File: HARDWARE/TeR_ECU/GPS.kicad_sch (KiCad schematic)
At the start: 11 parts, among them J5 GPS_ANT, U10 NEO-M9N

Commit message: Began layout
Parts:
- J5: footprint (none) -> Connector_Coaxial:SMA_Amphenol_132289_EdgeMount
- L2: footprint (none) -> Inductor_SMD:L_0805_2012Metric
- R45, R46: footprint (none) -> Resistor_SMD:R_0603_1608Metric
- TP1: footprint (none) -> TestPoint:TestPoint_Pad_1.0x1.0mm
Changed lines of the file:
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@@
 			)
 		)
-		(property "Footprint" ""
+		(property "Footprint" "Inductor_SMD:L_0805_2012Metric"
 			(at 161.29 85.09 0)
 			(effects
@@
 			)
 		)
-		(property "Footprint" ""
+		(property "Footprint" "Resistor_SMD:R_0603_1608Metric"
 			(at 144.78 115.57 0)
 			(effects
@@
 			)
 		)
-		(property "Footprint" ""
+		(property "Footprint" "Connector_Coaxial:SMA_Amphenol_132289_EdgeMount"
 			(at 191.77 92.71 0)
 			(effects
@@
 			)
 		)
-		(property "Footprint" ""
+		(property "Footprint" "Resistor_SMD:R_0603_1608Metric"
 			(at 163.068 77.47 90)
 			(effects
@@
 			)
 		)
-		(property "Footprint" ""
+		(property "Footprint" "TestPoint:TestPoint_Pad_1.0x1.0mm"
 			(at 92.71 100.33 0)
 			(effects

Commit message: First layout prototype
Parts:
- D25: footprint LED_SMD:LED_0201_0603Metric -> LED_SMD:LED_0603_1608Metric
- D26: footprint SODFL1006X40N -> GPS_D:SODFL1006X40N
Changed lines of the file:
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@@
 			)
 		)
-		(property "Footprint" "SODFL1006X40N"
+		(property "Footprint" "GPS_D:SODFL1006X40N"
 			(at 67.64 102.87 0)
 			(effects
@@
 			)
 		)
-		(property "Footprint" "LED_SMD:LED_0201_0603Metric"
+		(property "Footprint" "LED_SMD:LED_0603_1608Metric"
 			(at 144.78 106.68 0)
 			(effects

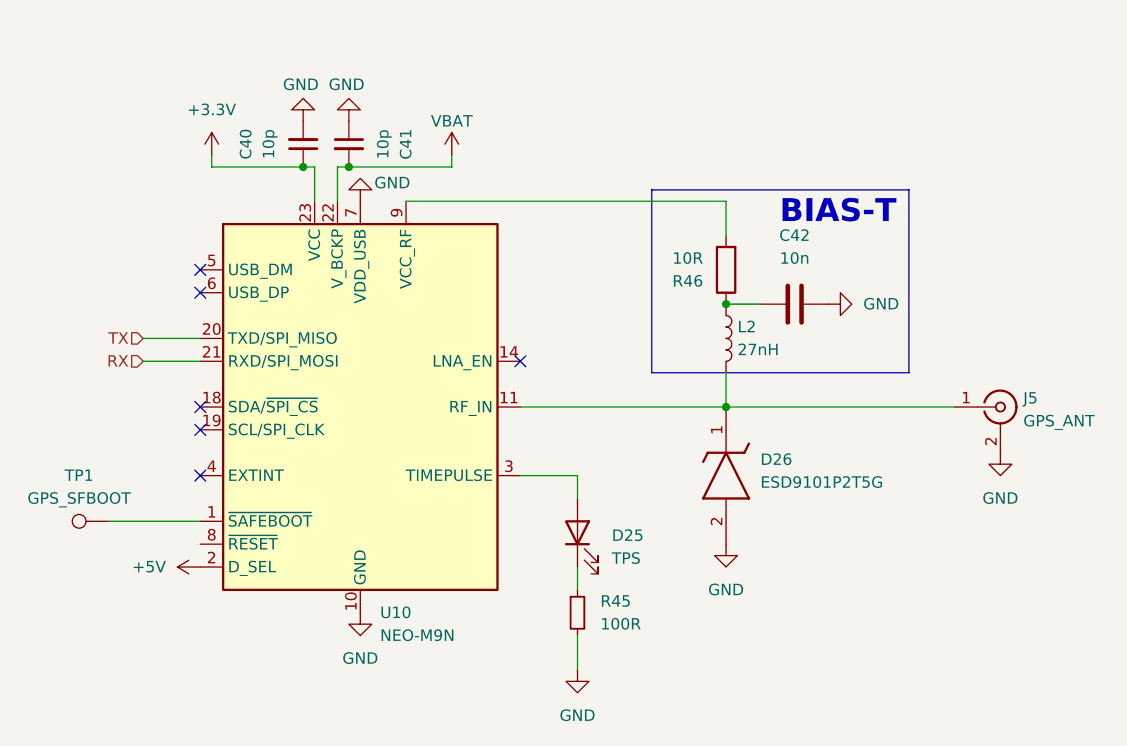
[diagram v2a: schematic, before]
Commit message: Finished layout, RF design, and quick DRC check, Lookin gud
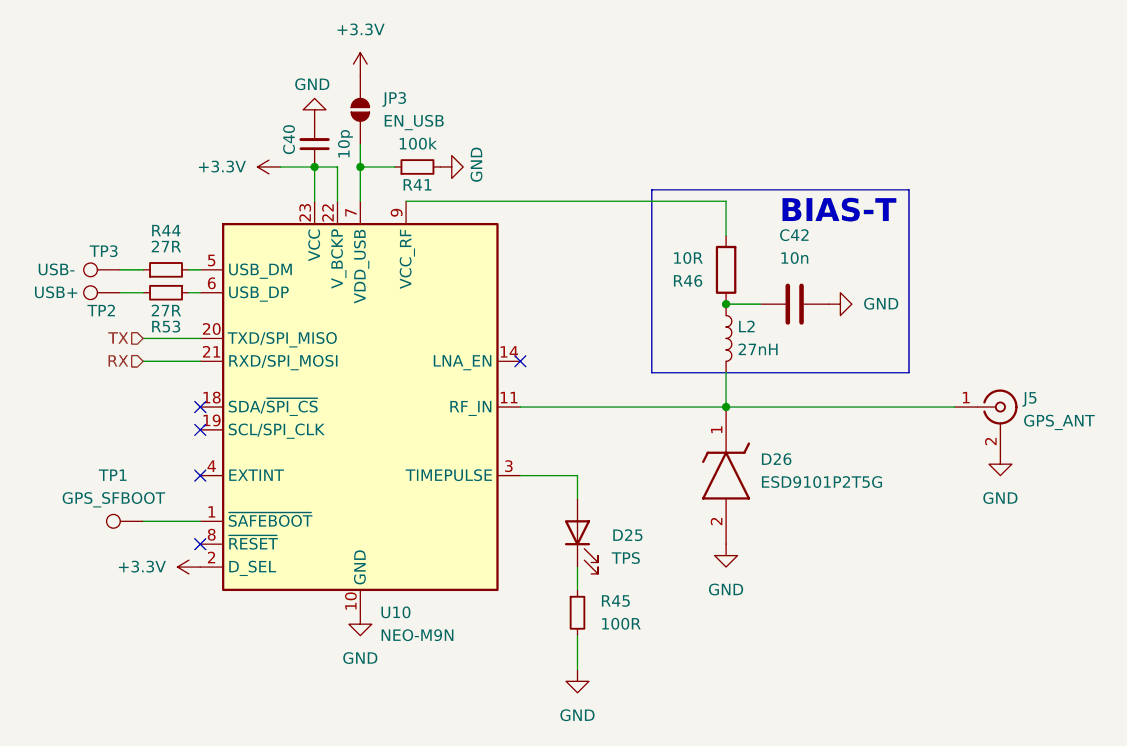
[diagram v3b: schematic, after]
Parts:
- removed C41: 10p, Capacitor_SMD:C_0603_1608Metric, symbol Device:C_Small
- added JP3: EN_USB, Jumper:SolderJumper-2_P1.3mm_Open_RoundedPad1.0x1.5mm, symbol Jumper:SolderJumper_2_Open
- added R41: 100k, Resistor_SMD:R_0603_1608Metric, symbol Device:R_Small
- added R44, R53: 27R, Resistor_SMD:R_0603_1608Metric, symbol Device:R_Small
- added TP2: USB+, TestPoint:TestPoint_Pad_1.0x1.0mm, symbol Connector:TestPoint
- added TP3: USB-, TestPoint:TestPoint_Pad_1.0x1.0mm, symbol Connector:TestPoint
- C42: footprint Capacitor_SMD:C_0603_1608Metric -> Capacitor_SMD:C_0402_1005Metric
- L2: footprint Inductor_SMD:L_0805_2012Metric -> Inductor_SMD:L_0402_1005Metric
- R46: footprint Resistor_SMD:R_0603_1608Metric -> Resistor_SMD:R_0402_1005Metric
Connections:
- net +5V is gone; now on net +3.3V: U10.2 (D_SEL)
- net VBAT is gone; now on net +3.3V: U10.22 (V_BCKP)
- net +3.3V: now also JP3.2 (B)
- net GND: now also R41.2; no longer U10.7 (VDD_USB)
- net at U10.5 (USB_DM): now also R44.2
- net at U10.6 (USB_DP): now also R53.1
- new net: R53.2, TP2.1
- new net: R44.1, TP3.1
- new net: JP3.1 (A), R41.1, U10.7 (VDD_USB)
- no-connect marks 6 -> 5
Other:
- moved on the sheet: C40, TP1
